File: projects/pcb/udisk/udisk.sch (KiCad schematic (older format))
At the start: 0 parts

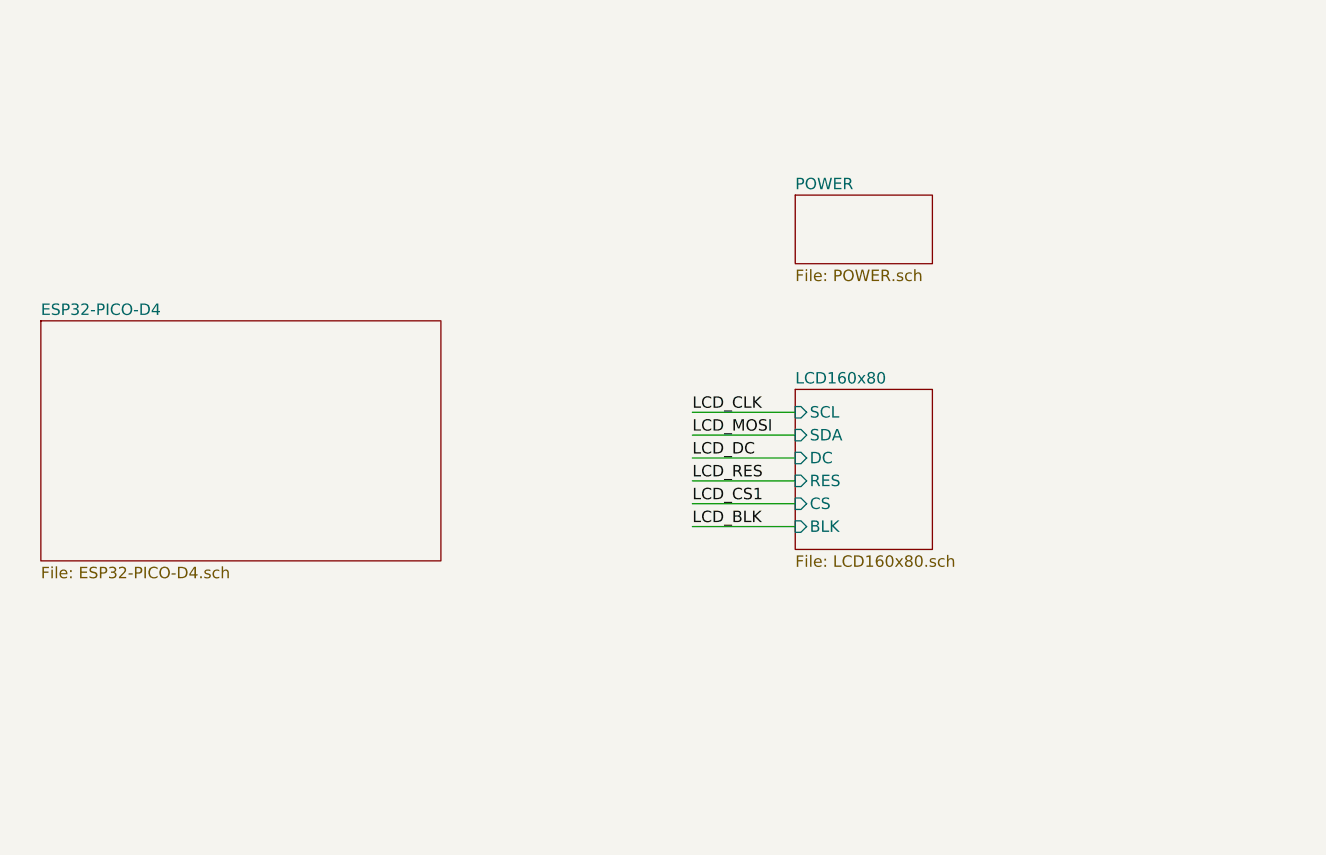
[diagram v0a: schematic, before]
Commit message: feature(pcb): pcb ok
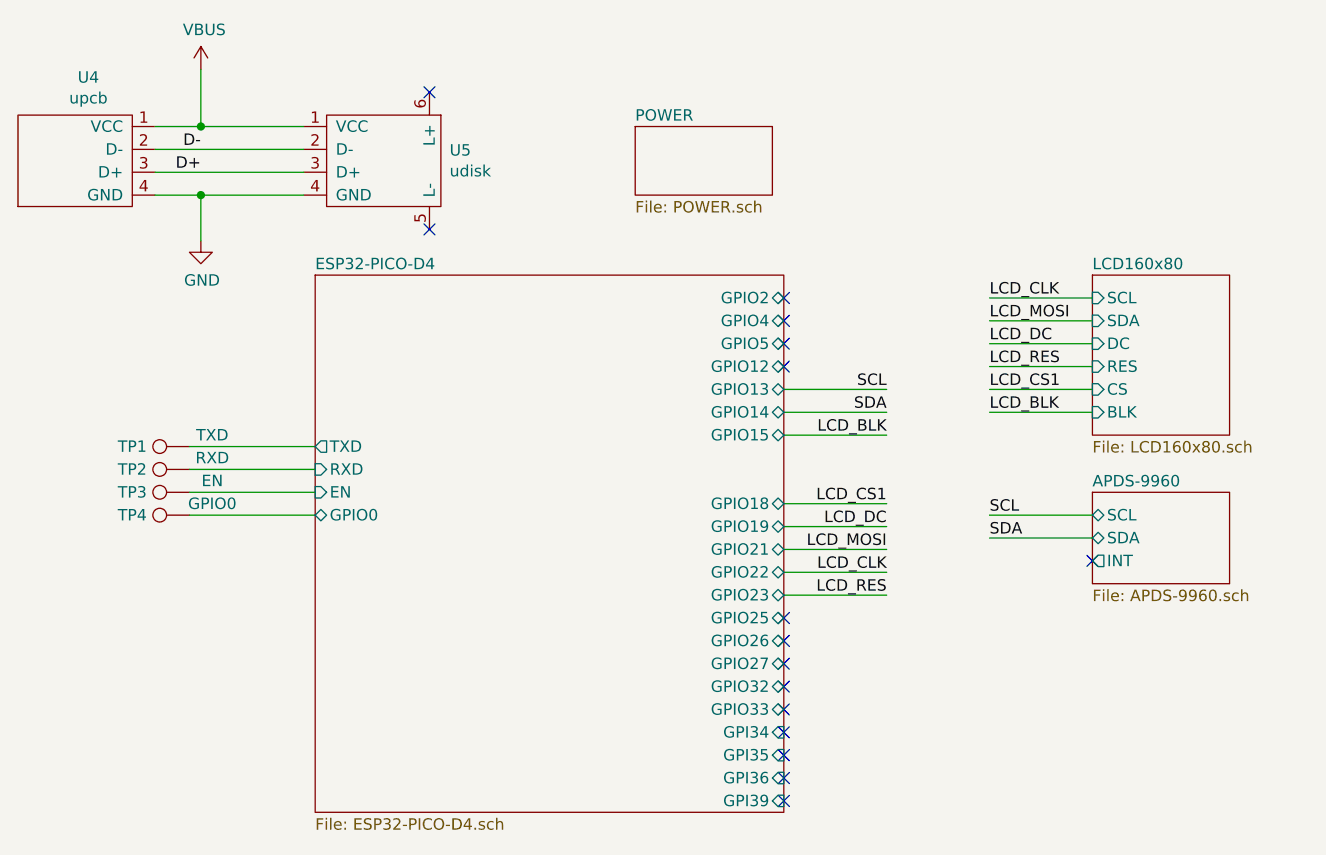
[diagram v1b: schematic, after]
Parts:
- added TP1: TXD, TestPoint:TestPoint_Pad_D1.0mm, symbol Connector:TestPoint
- added TP2: RXD, TestPoint:TestPoint_Pad_D1.0mm, symbol Connector:TestPoint
- added TP3: EN, TestPoint:TestPoint_Pad_D1.0mm, symbol Connector:TestPoint
- added TP4: GPIO0, TestPoint:TestPoint_Pad_D1.0mm, symbol Connector:TestPoint
- added U4: upcb, USB:upcb, symbol USB:upcb
- added U5: udisk, USB:udisk, symbol USB:udisk
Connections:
- new net D+: U4.3 (D+), U5.3 (D+)
- new net D-: U4.2 (D-), U5.2 (D-)
- new net ESP32-PICO-D4/EN: TP3.1
- new net ESP32-PICO-D4/GPIO0: TP4.1
- new net ESP32-PICO-D4/RXD: TP2.1
- new net ESP32-PICO-D4/TXD: TP1.1
- new net GND: U4.4 (GND), U5.4 (GND)
- new net VBUS: U4.1 (VCC), U5.1 (VCC)
- no-connect marks 0 -> 16
